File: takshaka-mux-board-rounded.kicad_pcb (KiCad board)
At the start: 2 copper layers, 30.3 x 24.2 mm, 10 parts, among them J1 Conn_01x01_Male, J2 Conn_01x01_Male, J3 Conn_02x08_Counter_Clockwise, J4 locked, U1 4051, U2 4051

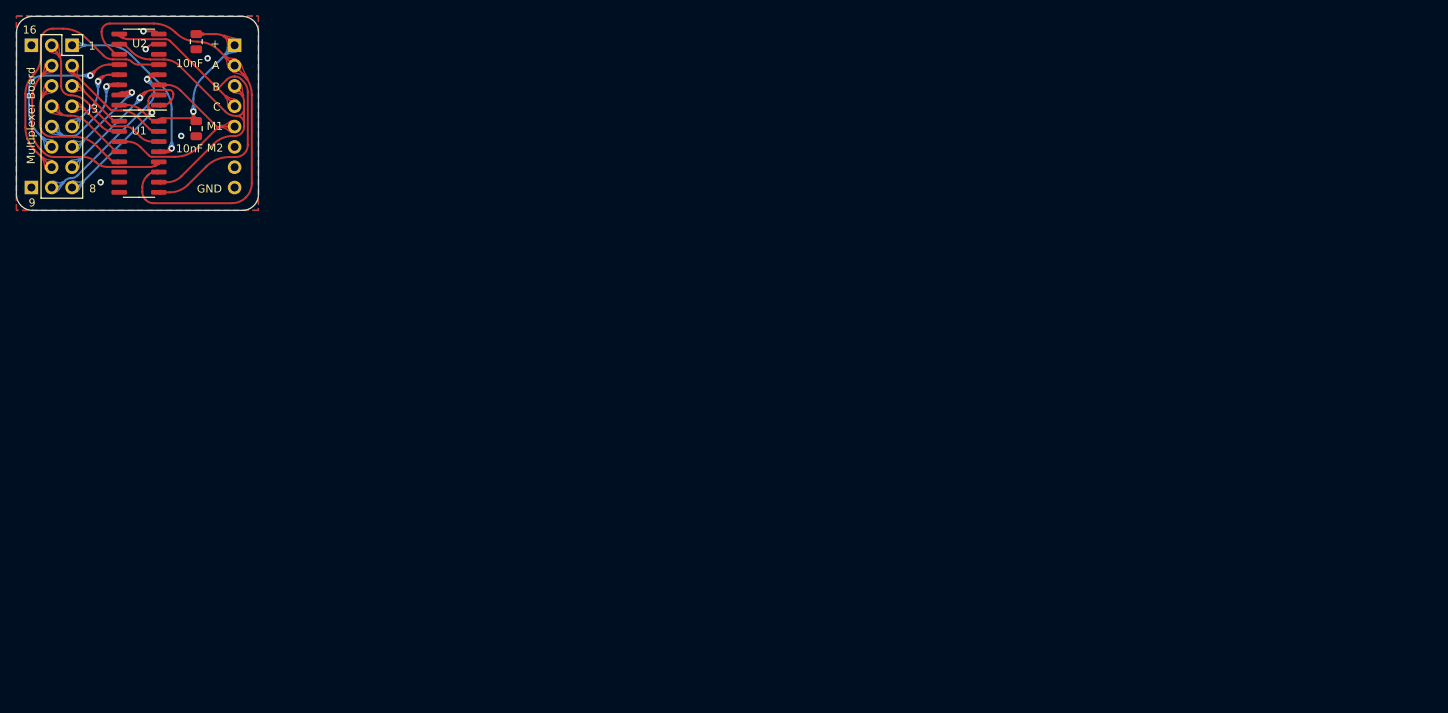
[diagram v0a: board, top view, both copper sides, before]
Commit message: rebuilt gerbers files.
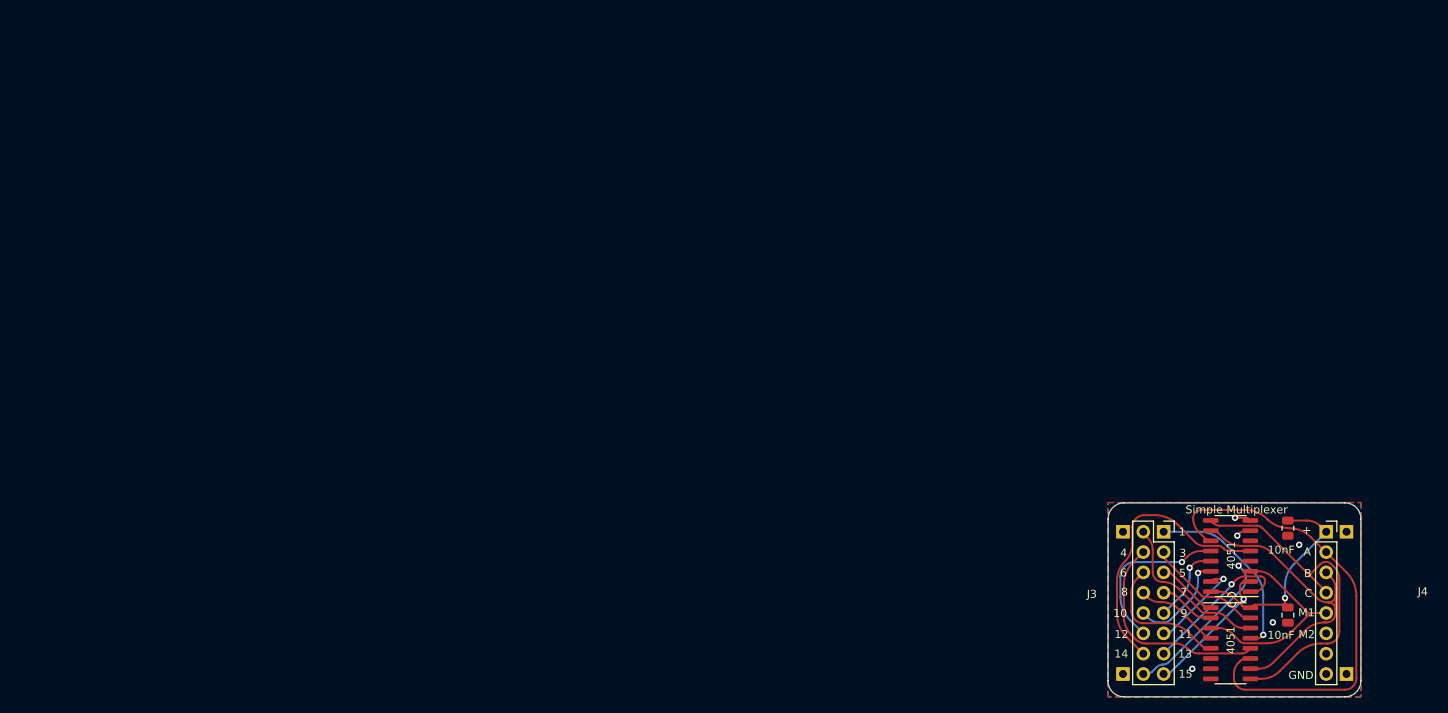
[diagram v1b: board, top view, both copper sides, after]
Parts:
- added J5: Conn_01x01_Male, Connector_PinHeader_2.54mm:PinHeader_1x01_P2.54mm_Vertical, B.Cu at (253.3, 152.2)
- added J6: Conn_01x01_Male, Connector_PinHeader_2.54mm:PinHeader_1x01_P2.54mm_Vertical, B.Cu at (225.3, 134.5)
- J4: footprint Connector_PinHeader_2.54mm:PinHeader_1x08_P2.54mm_Vertical -> Connector_PinSocket_2.54mm:PinSocket_1x08_P2.54mm_Vertical; moved to F.Cu
- moved J1 175.3 mm to (253.3, 134.5)
- moved G2 149.4 mm to (240.3, 134.6)
- moved U1 149.4 mm to (238.8, 148.4)
- moved U2 149.4 mm to (238.8, 137.5)
- moved C1 149.4 mm to (246.0, 134.0)
- moved C2 149.4 mm to (246.0, 144.9)
- moved G1 149.4 mm to (240.0, 148.0)
- moved J2 149.4 mm to (225.3, 152.2)
- moved J3 149.4 mm to (230.4, 134.5)
- moved J4 149.4 mm to (250.8, 134.5), turned to 0 degrees
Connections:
- net ATTACK renamed A
- net DECAY renamed D|R
- net DRIVE renamed D
- net P_D_MOD renamed PD_MOD
- net P_H_MOD renamed PH_MOD
- net P_S_MOD renamed PS_MOD
- net RES renamed R
- net RUMBLE renamed GROWL
- net SUSTAIN renamed S
- net S_C_MOD renamed SH_MOD
- net S_D_MOD renamed SD_MOD
- net S_S_MOD renamed SS_MOD
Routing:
- net CHANNEL_SELECT_A: track 57.7 -> 60.4 mm
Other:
- board size 30.3 x 24.2 mm -> 31.6 x 24.2 mm
- board text added: "10"
- board text added: "11"
- board text added: "12"
- board text added: "13"
- board text added: "14"
- board text added: "15"
- board text added: "2022.09.21 v0.2"
- board text added: "3"
- board text added: "4"
- board text added: "5"
- board text added: "6"
- board text added: "7"
- board text added: "Simple Multiplexer"
- board text removed: "16"
- board text removed: "2022.09.23 v0.1"
- board text removed: "Multiplexer Board"
